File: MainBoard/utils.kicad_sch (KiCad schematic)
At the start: 14 parts, among them Q1 AO3400A, U3 LIS3DH

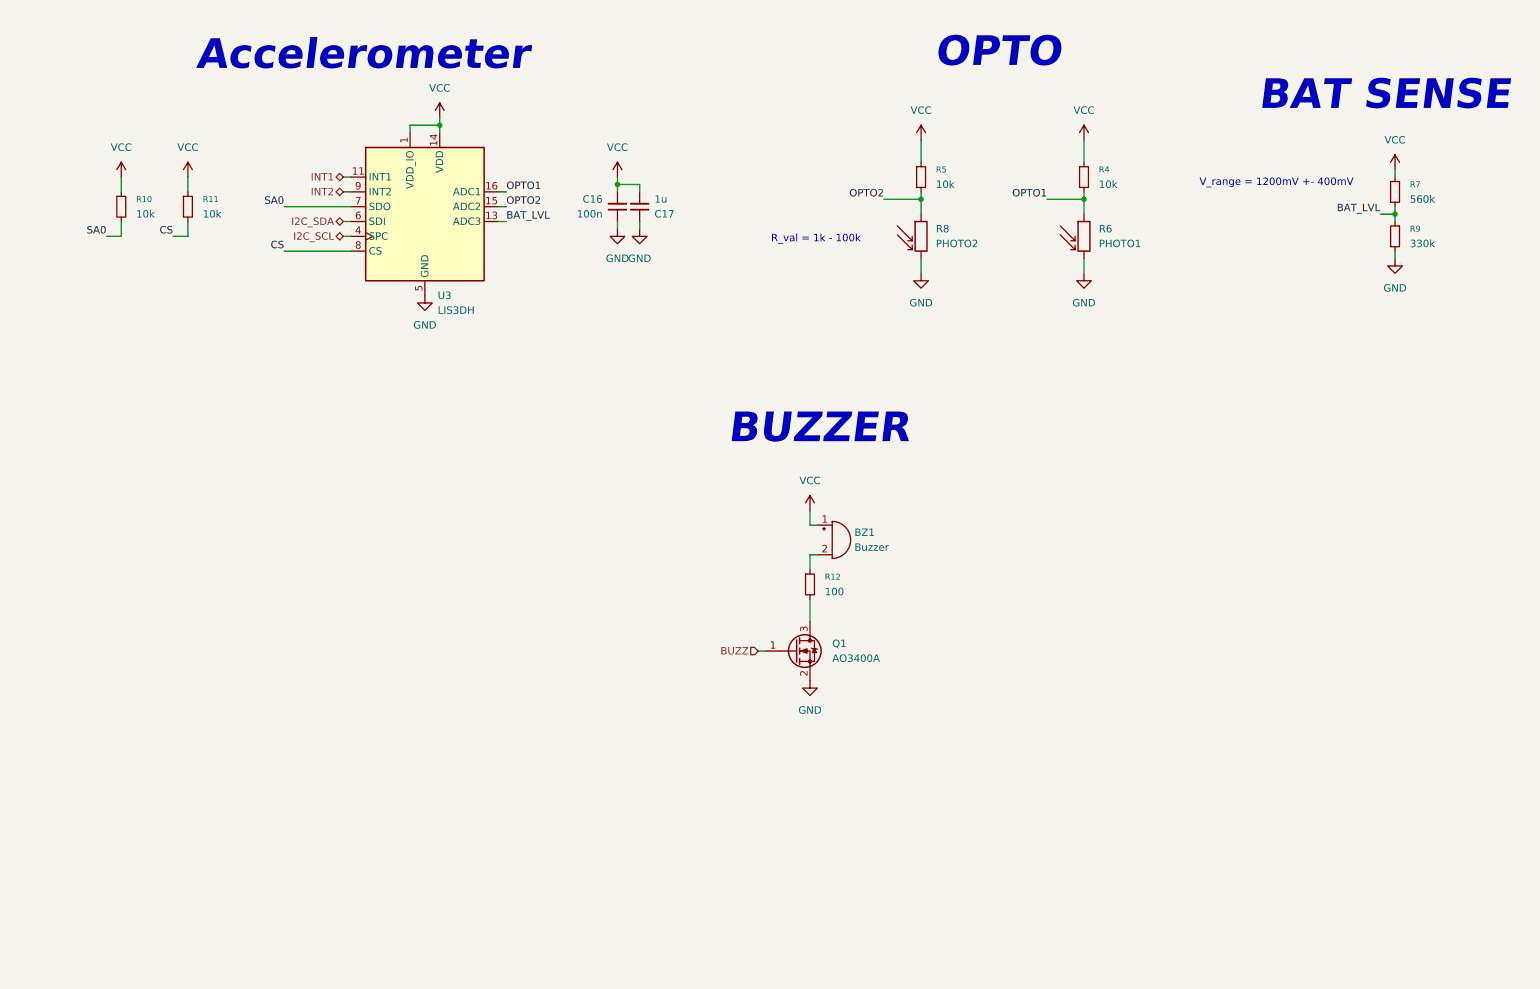
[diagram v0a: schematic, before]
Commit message: change schematic
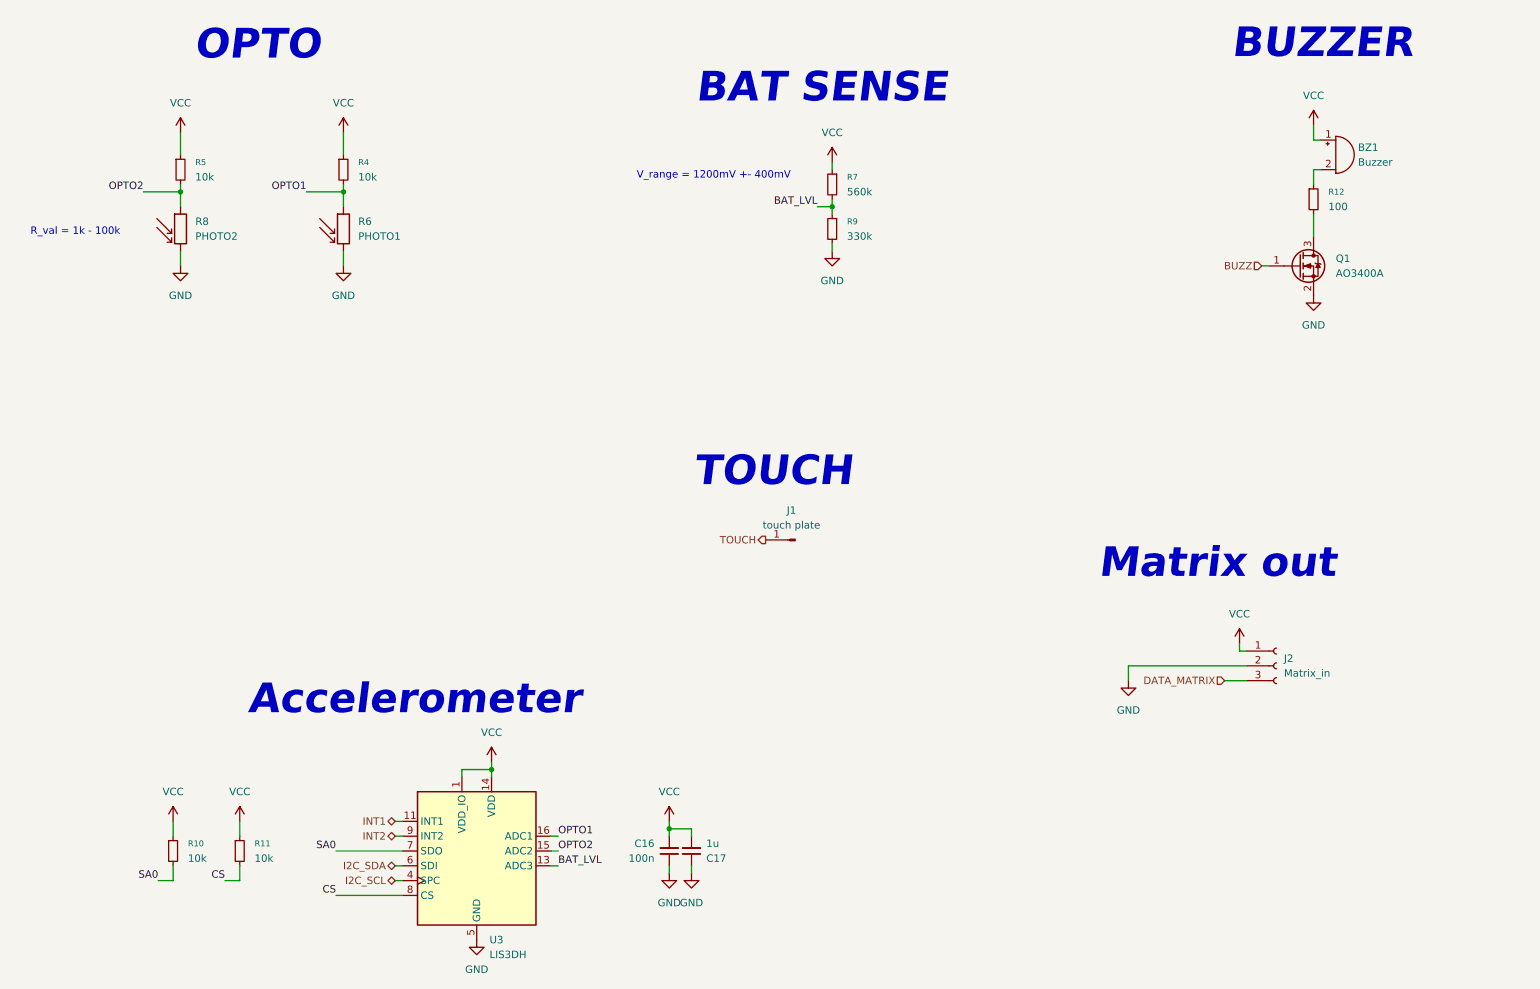
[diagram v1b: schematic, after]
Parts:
- added J1: touch plate, Connector_Pin:Pin_D1.0mm_L10.0mm, symbol Connector:Conn_01x01_Pin
- added J2: Matrix_in, Connector_PinSocket_2.54mm:PinSocket_1x03_P2.54mm_Vertical, symbol Connector:Conn_01x03_Socket
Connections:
- net GND: now also J2.2 (Pin_2)
- net VCC: now also J2.1 (Pin_1)
- new net DATA_MATRIX: J2.3 (Pin_3)
- new net TOUCH: J1.1 (Pin_1)
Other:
- note added: "Matrix out"
- note added: "TOUCH"
- moved on the sheet: BZ1, C16, C17, Q1, R10, R11, R12, R4, R5, R6, R7, R8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
